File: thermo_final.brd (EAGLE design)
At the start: 69.4 x 89 mm, 109 parts, among them IC1 DG4051EEQ-T1-GE3, IC2 DG4051EEQ-T1-GE3, IC5 MAX6675ISA+

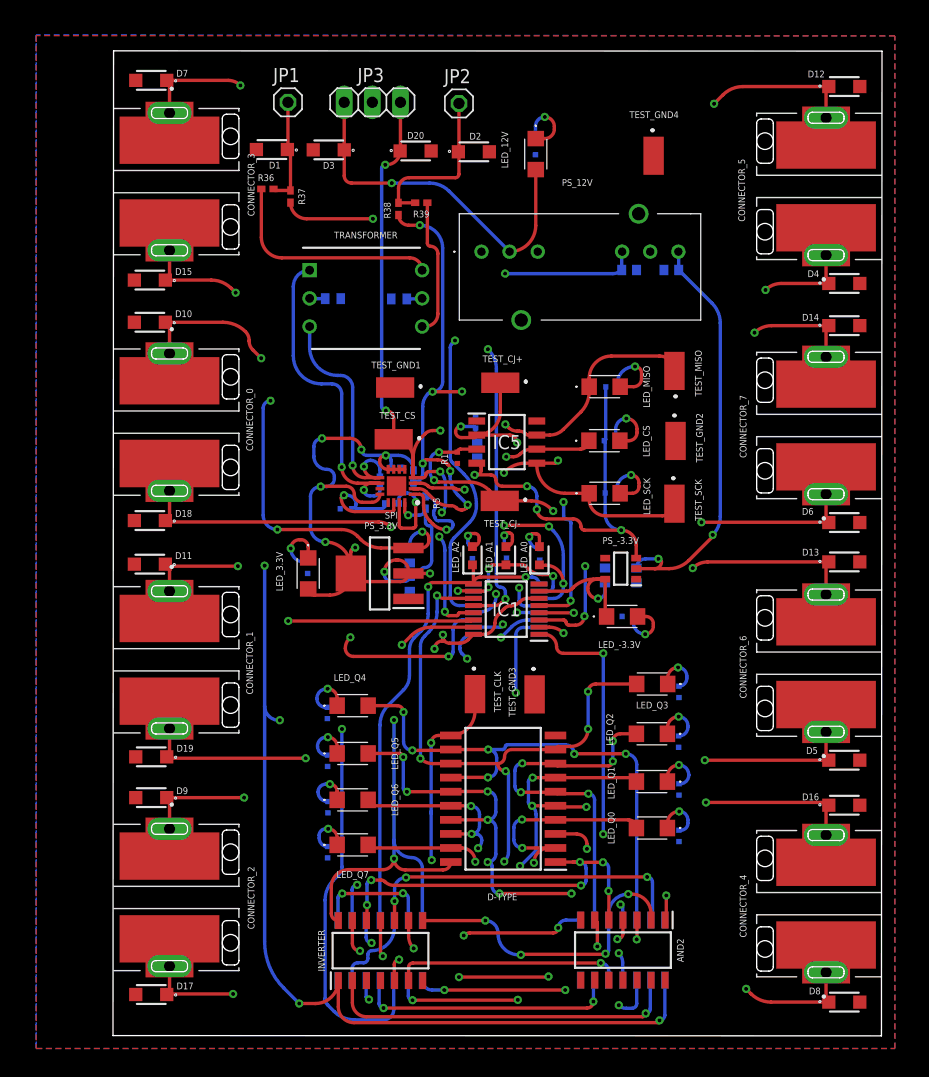
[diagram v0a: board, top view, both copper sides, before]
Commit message: Board Complete
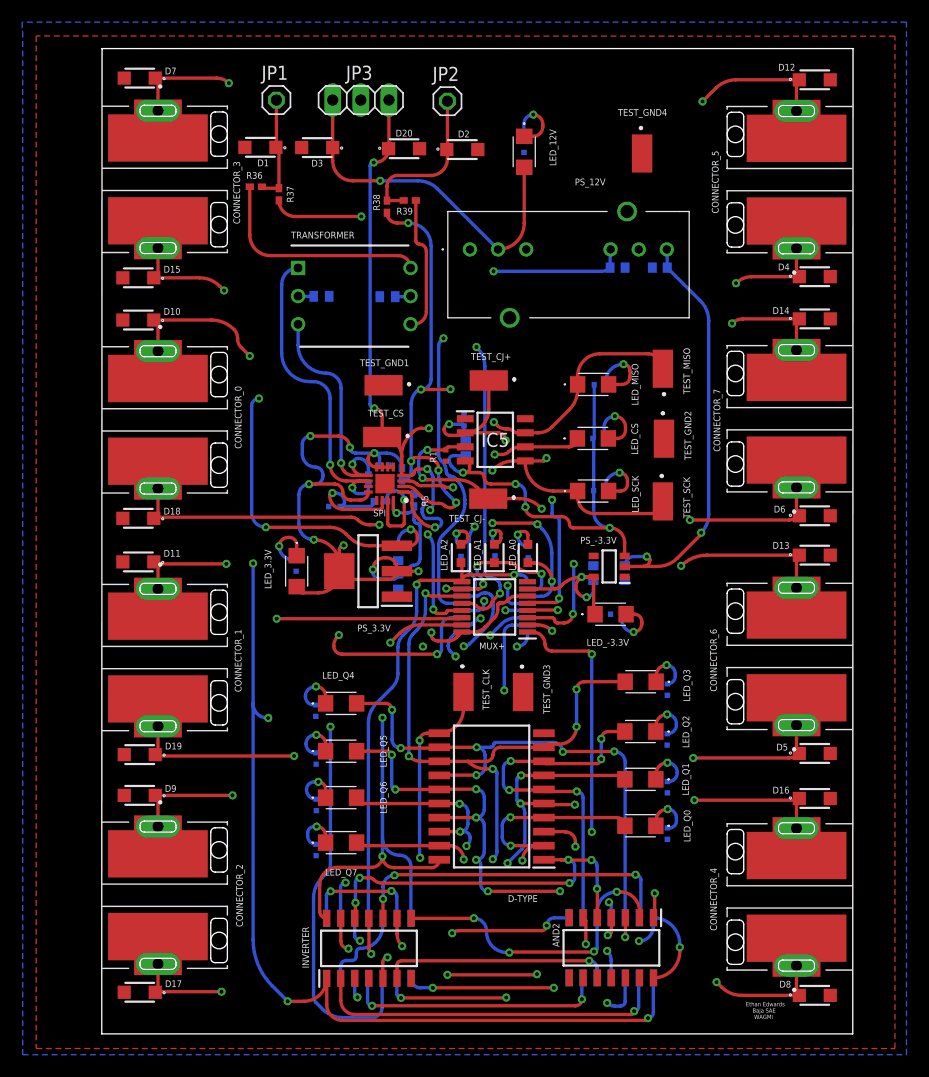
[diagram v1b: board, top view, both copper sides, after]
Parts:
- removed IC1, IC2: DG4051EEQ-T1-GE3, SamacSys_Parts:SOP65P640X120-16N
- added MUX+, MUX-: DG4051EEQ-T1-GE3, SamacSys_Parts:SOP65P640X120-16N
- moved D14 2.74 mm to (64.4, 64.4)
- moved CONNECTOR_4 2.74 mm to (62.7, 12.2)
- moved CONNECTOR_5 2.74 mm to (62.7, 77.0)
- moved CONNECTOR_6 2.74 mm to (62.7, 34.0)
- moved CONNECTOR_7 2.74 mm to (62.7, 55.4)
- moved D12 2.74 mm to (64.4, 86.0)
- moved D13 2.74 mm to (64.4, 43.1)
- moved D16 2.74 mm to (64.4, 21.1)
- moved D4 2.74 mm to (64.4, 68.2)
- moved D5 2.74 mm to (64.4, 25.2)
- moved D6 2.74 mm to (64.4, 46.7)
- moved D8 2.74 mm to (64.4, 3.35)
- moved C3 1.06 mm to (46.6, 69.1)
- moved C4 1.06 mm to (50.4, 69.1)
- moved JP2 1.06 mm to (31.2, 84.1)
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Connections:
- net -VCC: now also MUX+.7, MUX-.7; no longer IC1.7, IC2.7
- net A1: now also MUX+.10, MUX-.10; no longer IC1.10, IC2.10
- net A2: now also MUX+.9, MUX-.9; no longer IC1.9, IC2.9
- net CJ+: now also MUX+.3; no longer IC1.3
- net CJ-: now also MUX-.3; no longer IC2.3
- net GND: now also MUX+.8, MUX-.8; no longer IC1.8, IC2.8
- net Q3: now also MUX+.11, MUX-.11; no longer IC1.11, IC2.11
- net T0+: now also MUX+.13; no longer IC1.13
- net T0-: now also MUX-.13; no longer IC2.13
- net T1+: now also MUX+.14; no longer IC1.14
- net T1-: now also MUX-.14; no longer IC2.14
- net T2+: now also MUX+.15; no longer IC1.15
- net T2-: now also MUX-.15; no longer IC2.15
- net T3+: now also MUX+.12; no longer IC1.12
- net T3-: now also MUX-.12; no longer IC2.12
- net T4+: now also MUX+.1; no longer IC1.1
- net T4-: now also MUX-.1; no longer IC2.1
- net T5+: now also MUX+.5; no longer IC1.5
- net T5-: now also MUX-.5; no longer IC2.5
- net T6+: now also MUX+.2; no longer IC1.2
- net T6-: now also MUX-.2; no longer IC2.2
- net T7+: now also MUX+.4; no longer IC1.4
- net T7-: now also MUX-.4; no longer IC2.4
- net VCC: now also MUX+.16, MUX+.6, MUX-.16, MUX-.6; no longer IC1.16, IC1.6, IC2.16, IC2.6
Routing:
- net VCC: track 181.1 -> 248.7 mm, vias 17 -> 21
- net -VCC: track 14.5 -> 33.2 mm, vias 1 -> 3
- net T4-: track 43.8 -> 42.1 mm
- net T7+: track 32.1 -> 30.4 mm
- net T6+: track 33.5 -> 32.0 mm
- net T4+: track 52.6 -> 51.2 mm
- net T6-: track 36.8 -> 35.4 mm
- net T5-: track 72.9 -> 71.6 mm
- net Q3: track 90.9 -> 92.2 mm
- net T3+: track 69.4 -> 70.6 mm
- net N$40: track 15.3 -> 14.6 mm
- net VDD: track 32.6 -> 32.0 mm
- net T5+: track 47.3 -> 46.7 mm
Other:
- board size 69.4 x 89 mm -> 67.8 x 89 mm
- board text added: "Ethan Edwards Baja SAE WAGMI"
